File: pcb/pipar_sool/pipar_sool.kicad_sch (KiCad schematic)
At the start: 46 parts, among them SW1 SW_Wuerth_450301014042, U1 Seeeduino Xiao nRF52840

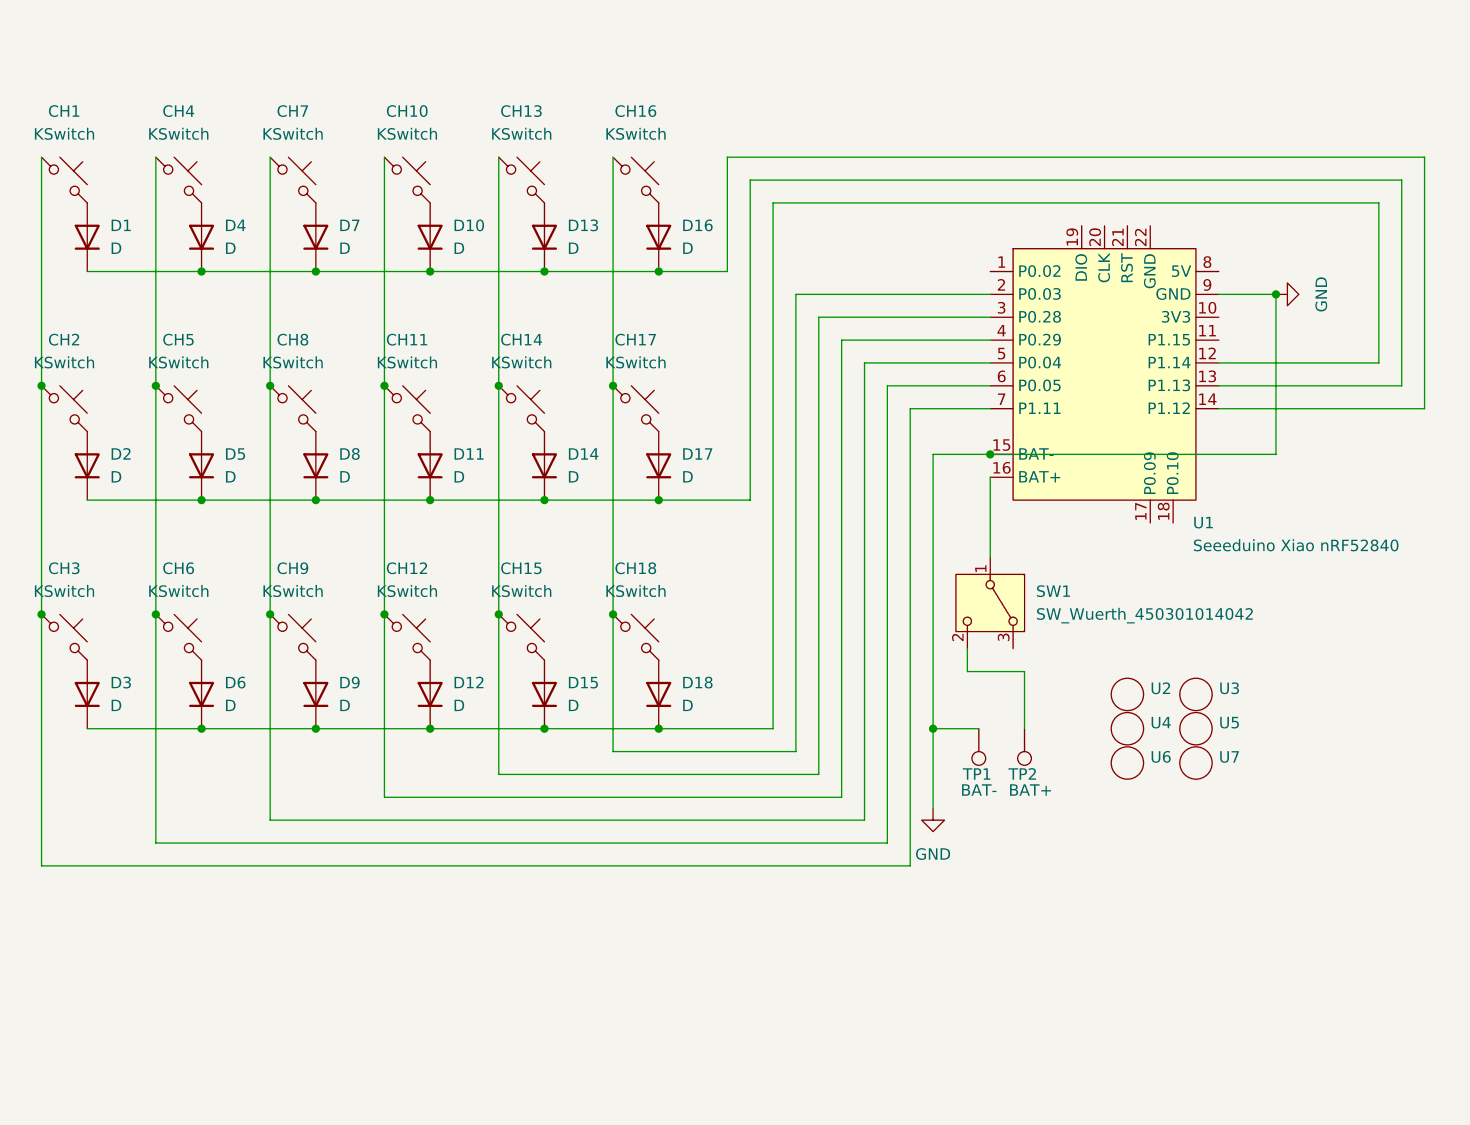
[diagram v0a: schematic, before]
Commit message: start of creating newer models
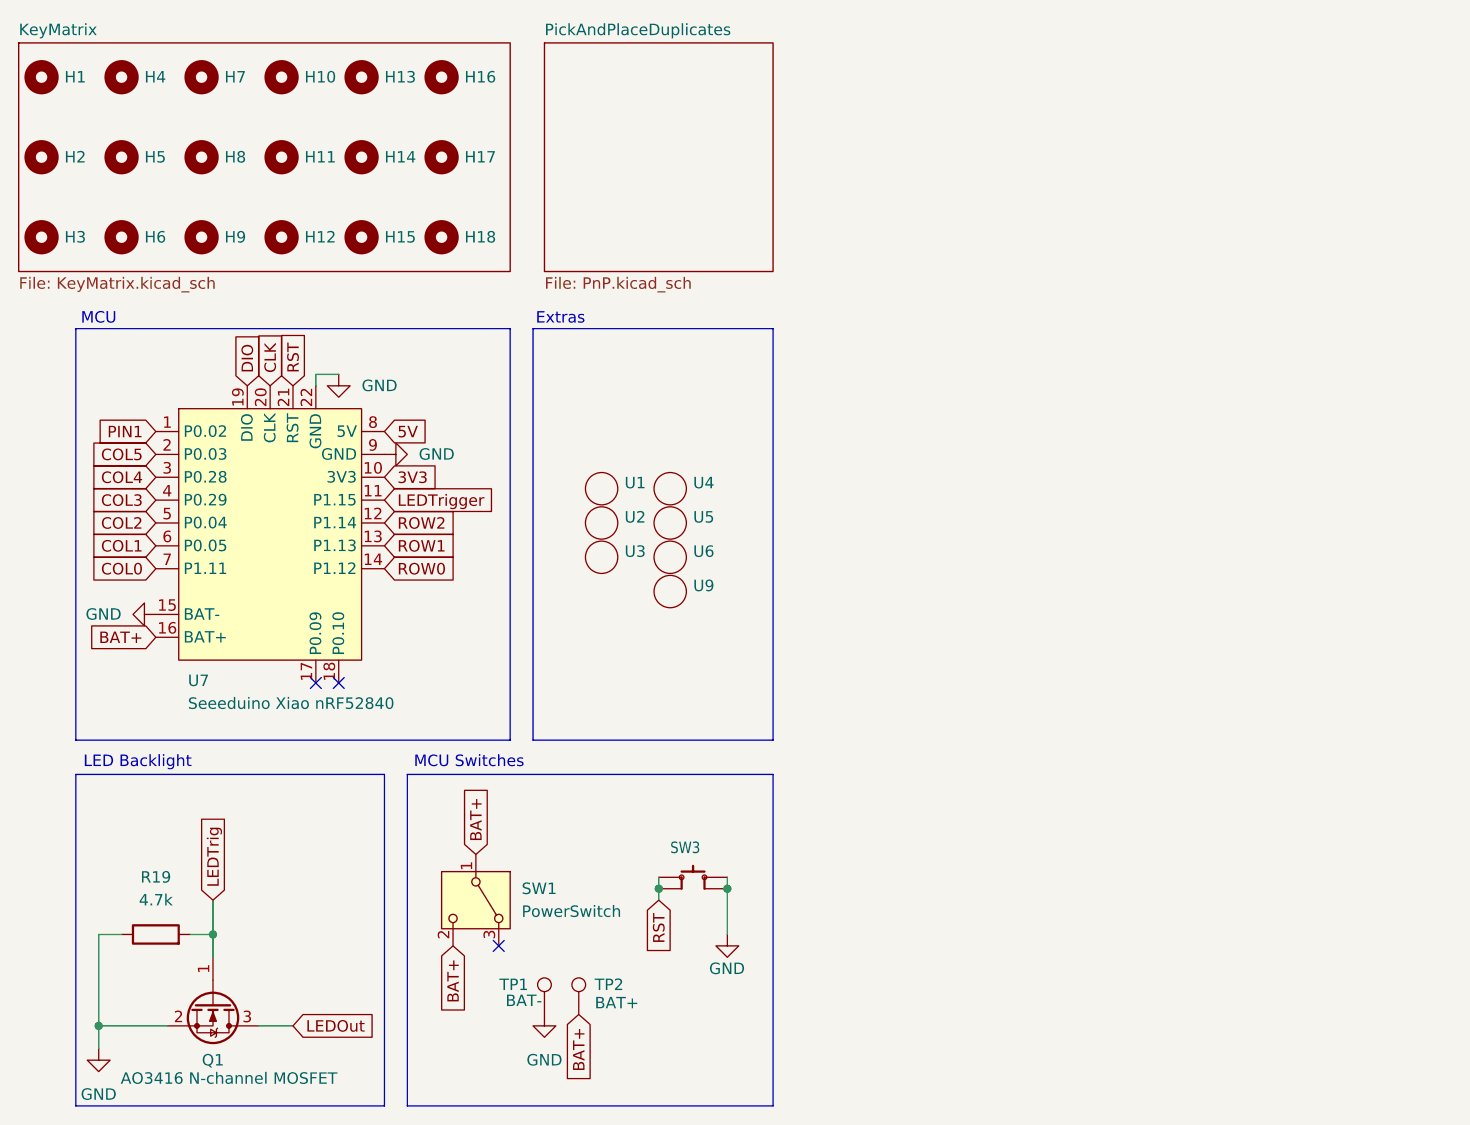
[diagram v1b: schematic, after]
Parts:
- removed CH1, CH10, CH11, CH12, CH13, CH14, CH15, CH16, CH17, CH18, CH2, CH3, CH4, CH5, CH6, CH7, CH8, CH9: KSwitch, keyswitches:Kailh_socket_PG1350_reversible, symbol marbastlib-choc:choc_v1_SW_HS_CPG135001S30
- removed D1, D10, D11, D12, D13, D14, D15, D16, D17, D18, D2, D3, D4, D5, D6, D7, D8, D9: D, Diode_SMD:Nexperia_CFP3_SOD-123W, symbol Device:D
- removed U1: Seeeduino Xiao nRF52840, Seeed Studio XIAO Series Library:XIAO-nRF52840-Sense-14P-2.54-21X17.8MM, symbol marbastlib-promicroish:Seeeduino_Xiao_nRF52840
- removed U7: ~, Art:Salt, symbol Trackpoint:Solder_Nut
- added H1, H10, H11, H12, H13, H14, H15, H16, H17, H18, H2, H3, H4, H5, H6, H7, H8, H9: MountingHole, Keyboard:Kailh_socket_PG1350_reversible_Holes, symbol Mechanical:MountingHole
- added Q1: AO3416 N-channel MOSFET, Package_TO_SOT_SMD:SOT-23, symbol Device:Q_NMOS_GSD
- added R19: 4.7k, Resistor_SMD:R_0402_1005Metric_Pad0.72x0.64mm_HandSolder, symbol PCM_4ms_Resistor:10m_1206_250mW
- added SW3: BUTTON-4P, Keyboard:SW4-SMD-2.8-2.6X1.6X0.53MM, symbol Seeed Studio XIAO nRF52840 v1.1-eagle-import:BUTTON-4P
- added U1: ~, Keyboard:Solder Nut, symbol Trackpoint:Solder_Nut
- added U7: Seeeduino Xiao nRF52840, Keyboard:XIAO-nRF52840-Sense-14P-2.54-21X17.8MM, symbol xiao_ble:Seeeduino_Xiao_nRF52840
- added U9: ~, Art:Salt, symbol Trackpoint:Solder_Nut
- SW1: value SW_Wuerth_450301014042 -> PowerSwitch
- U2, U3, U4, U5: footprint MountingHole:MountingHole_2.2mm_M2 -> Keyboard:Solder Nut
- U6: footprint MountingHole:MountingHole_2.2mm_M2 -> Art:Salt; now left out of the parts list
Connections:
- net GND: now also Q1.2 (S), R19.1, SW3.2 (B0), SW3.4 (B1), U7.15 (BAT-), U7.22 (GND), U7.9 (GND)
- net BAT+: now reaches SW1.2 (C), TP2.1
- net BAT+: now also SW1.1 (B), U7.16 (BAT+)
- new net 3V3: U7.10 (3V3)
- new net 5V: U7.8 (5V)
- new net CLK: U7.20 (CLK)
- new net COL0: U7.7 (P1.11)
- new net COL1: U7.6 (P0.05)
- new net COL2: U7.5 (P0.04)
- new net COL3: U7.4 (P0.29)
- new net COL4: U7.3 (P0.28)
- new net COL5: U7.2 (P0.03)
- new net DIO: U7.19 (DIO)
- new net LEDOut: Q1.3 (D)
- new net LEDTrig: Q1.1 (G), R19.2
- new net LEDTrigger: U7.11 (P1.15)
- new net PIN1: U7.1 (P0.02)
- new net ROW0: U7.14 (P1.12)
- new net ROW1: U7.13 (P1.13)
- new net ROW2: U7.12 (P1.14)
- new net RST: SW3.1 (A0), SW3.3 (A1), U7.21 (RST)
- no-connect marks 0 -> 3
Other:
- added sheet KeyMatrix (KeyMatrix.kicad_sch)
- added sheet PickAndPlaceDuplicates (PnP.kicad_sch)
- note added: "Extras"
- note added: "LED Backlight"
- note added: "MCU"
- note added: "MCU Switches"

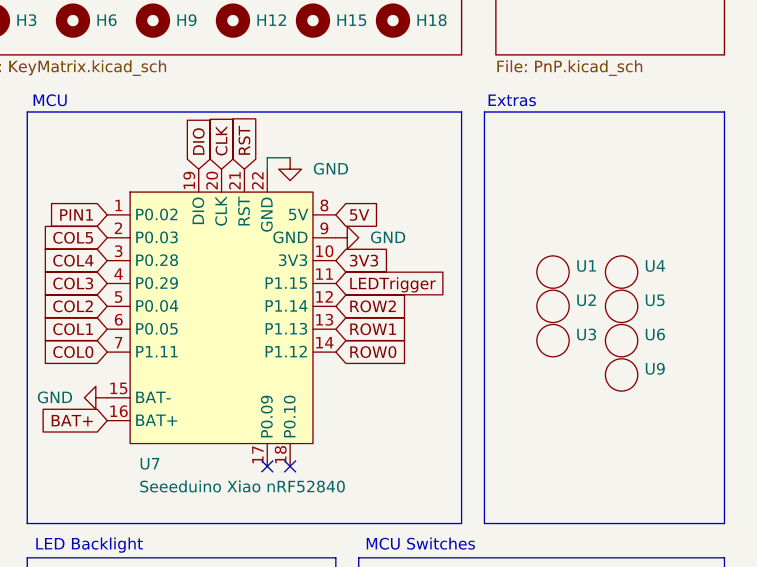
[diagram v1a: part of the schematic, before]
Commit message: add changes
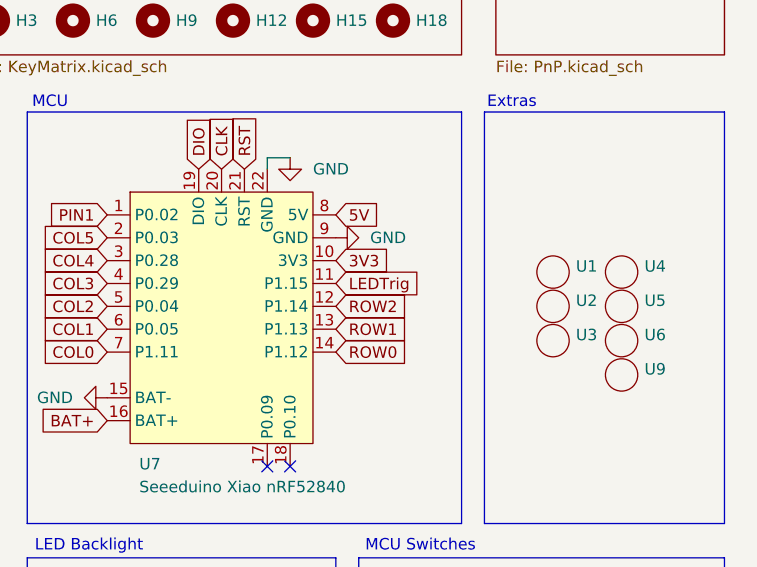
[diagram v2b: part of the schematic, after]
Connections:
- net LEDTrigger is gone; now on net LEDTrig: U7.11 (P1.15)
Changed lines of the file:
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@@
-		)
-	)
-	(global_label "LEDTrigger"
-		(shape input)
-		(at 53.34 66.04 0)
-		(fields_autoplaced yes)
-		(effects
-			(font
-				(size 1.27 1.27)
-			)
-			(justify left)
-		)
-		(property "Intersheetrefs" "${INTERSHEET_REFS}"
-			(at 66.3037 66.04 0)
-			(effects
-				(font
-					(size 1.27 1.27)
-				)
-				(justify left)
-				(hide yes)
-			)
 		)
 	)
@@
 			(effects
 				(font
+					(size 1.27 1.27)
+				)
+				(justify left)
+				(hide yes)
+			)
+		)
+	)
+	(global_label "LEDTrig"
+		(shape input)
+		(at 53.34 66.04 0)
+		(fields_autoplaced yes)
+		(effects
+			(font
+				(size 1.27 1.27)
+			)
+			(justify left)
+		)
+		(property "Intersheetrefs" "${INTERSHEET_REFS}"
+			(at 63.2799 66.04 0)
+			(effects
+				(font

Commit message: Remove obsolete files and update KiCad project settings for compatibility
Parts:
- U6, U9: footprint Art:Salt -> Art:Salt-smallest
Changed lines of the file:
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@@
 (kicad_sch
-	(version 20231120)
+	(version 20250114)
 	(generator "eeschema")
-	(generator_version "8.0")
+	(generator_version "9.0")
 	(paper "A4")
+	(rectangle
+		(start 19.05 96.52)
+		(end 53.34 133.35)
+		(stroke
+			(width 0)
+			(type default)
+		)
+		(fill
+			(type none)
+		)
+	)
+	(rectangle
+		(start 19.05 46.99)
+		(end 67.31 92.71)
+		(stroke
+			(width 0)
+			(type default)
+		)
+		(fill
+			(type none)
+		)
+	)
+	(rectangle
+		(start 69.85 46.99)
+		(end 96.52 92.71)
+		(stroke
+			(width 0)
+			(type default)
+		)
+		(fill
+			(type none)
+		)
+	)
+	(rectangle
+		(start 55.88 96.52)
+		(end 96.52 133.35)
+		(stroke
+			(width 0)
+			(type default)
+		)
+		(fill
+			(type none)
+		)
+	)
+	(text "LED Backlight"
+		(exclude_from_sim no)
+		(at 25.908 95.25 0)
+		(effects
+			(font
+				(size 1.27 1.27)
+			)
+		)
+	)
+	(text "MCU Switches"
+		(exclude_from_sim no)
+		(at 62.738 95.25 0)
+		(effects
+			(font
+				(size 1.27 1.27)
+			)
+		)
+	)
+	(text "MCU"
+		(exclude_from_sim no)
+		(at 21.59 45.974 0)
+		(effects
+			(font
+				(size 1.27 1.27)
+			)
+		)
+	)
+	(text "Extras"
+		(exclude_from_sim no)
+		(at 72.898 45.974 0)
+		(effects
+			(font
+				(size 1.27 1.27)
+			)
+		)
+	)
 	(junction
 		(at 83.82 109.22)
@@
 		)
 	)
-	(rectangle
-		(start 19.05 96.52)
-		(end 53.34 133.35)
-		(stroke
-			(width 0)
-			(type default)
-		)
-		(fill
-			(type none)
-		)
-	)
-	(rectangle
-		(start 19.05 46.99)
-		(end 67.31 92.71)
-		(stroke
-			(width 0)
-			(type default)
-		)
-		(fill
-			(type none)
-		)
-	)
-	(rectangle
-		(start 69.85 46.99)
-		(end 96.52 92.71)
-		(stroke
-			(width 0)
-			(type default)
-		)
-		(fill
-			(type none)
-		)
-	)
-	(rectangle
-		(start 55.88 96.52)
-		(end 96.52 133.35)
-		(stroke
-			(width 0)
-			(type default)
-		)
-		(fill
-			(type none)
-		)
-	)
-	(text "LED Backlight"
-		(exclude_from_sim no)
-		(at 25.908 95.25 0)
-		(effects
-			(font
-				(size 1.27 1.27)
-			)
-		)
-	)
-	(text "MCU Switches"
-		(exclude_from_sim no)
-		(at 62.738 95.25 0)
-		(effects
-			(font
-				(size 1.27 1.27)
-			)
-		)
-	)
-	(text "MCU"
-		(exclude_from_sim no)
-		(at 21.59 45.974 0)
-		(effects
-			(font
-				(size 1.27 1.27)
-			)
-		)
-	)
-	(text "Extras"
-		(exclude_from_sim no)
-		(at 72.898 45.974 0)
-		(effects
-			(font
-				(size 1.27 1.27)
-			)
-		)
-	)
 	(global_label "LEDTrig"
 		(shape input)
@@
 			)
 		)
-		(property "Footprint" "Art:Salt"
+		(property "Footprint" "Art:Salt-smallest"
 			(at 85.09 72.39 0)
 			(effects
@@
 			)
 		)
-		(property "Footprint" "Art:Salt"
+		(property "Footprint" "Art:Salt-smallest"
 			(at 85.09 76.2 0)
 			(effects
@@
 		(at 71.12 15.24)
 		(size 25.4 25.4)
+		(exclude_from_sim no)
+		(in_bom yes)
+		(on_board yes)
+		(dnp no)
 		(fields_autoplaced yes)
 		(stroke
@@
 		(at 12.7 15.24)
 		(size 54.61 25.4)
+		(exclude_from_sim no)
+		(in_bom yes)
+		(on_board yes)
+		(dnp no)
 		(fields_autoplaced yes)
 		(stroke
@@
 		)
 	)
+	(embedded_fonts no)
 )
